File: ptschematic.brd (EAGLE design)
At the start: 33.5 x 51.6 mm, 26 parts, among them U3 NCP1117LPST33T3G, U4 BGM13S, Y2 32MHz

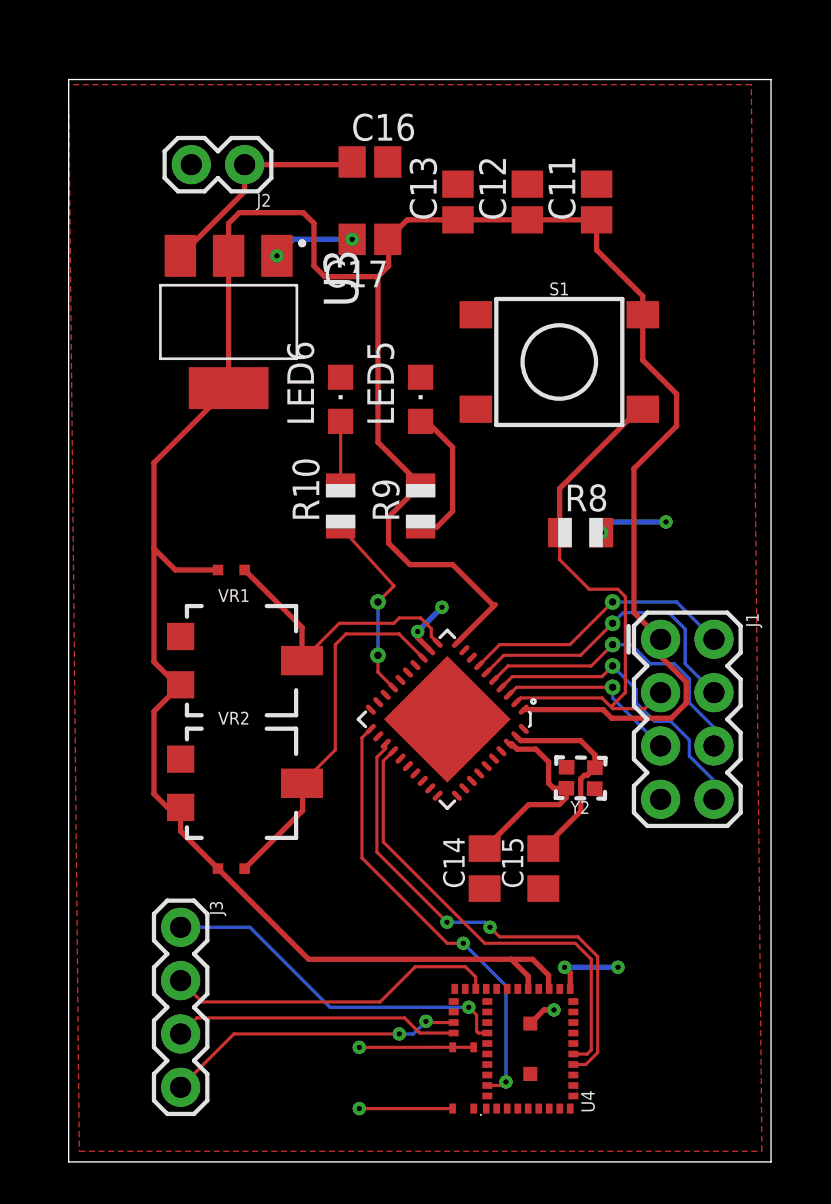
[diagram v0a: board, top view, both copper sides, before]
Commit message: Final Board and Gerber files
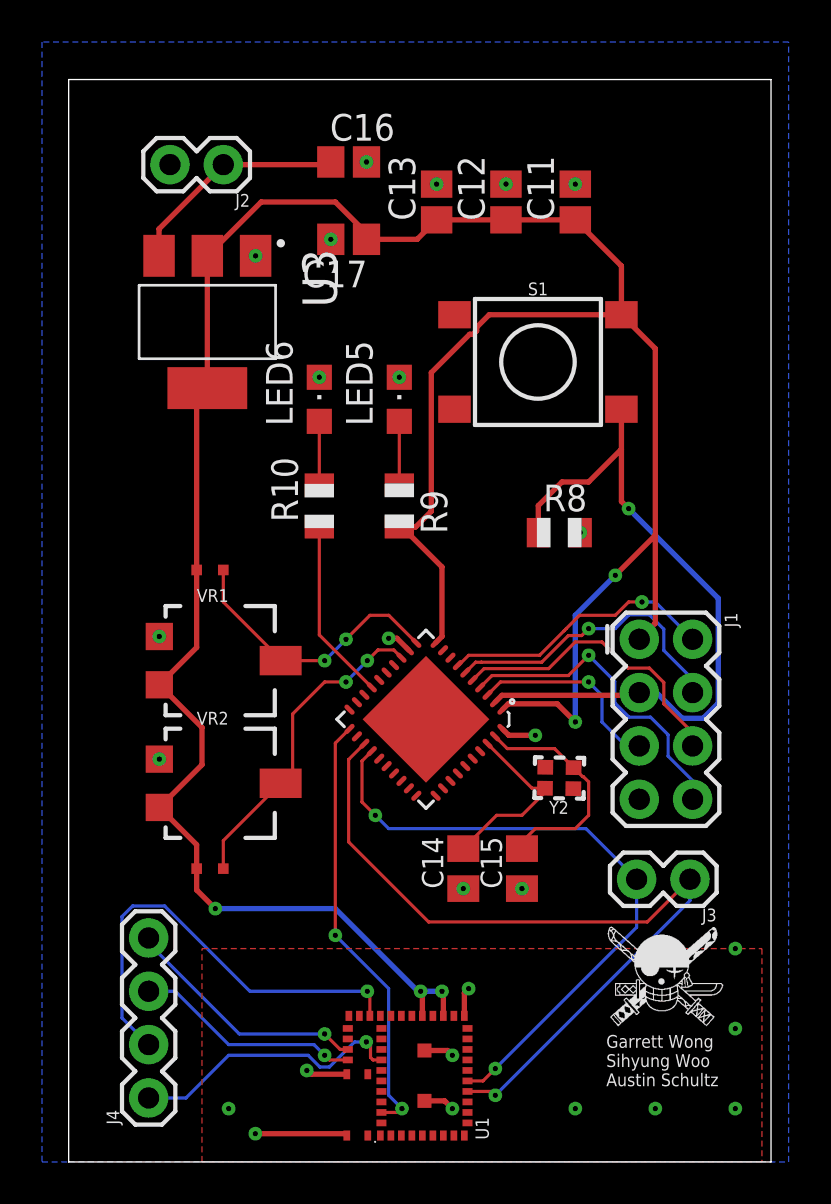
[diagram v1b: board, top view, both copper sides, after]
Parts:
- removed U4: BGM13S, BMES-Spr2019:BGM13S
- added J4: (no value), SparkFun-Connectors:1X04
- added U1: BGM13S, BMES-Spr2019:BGM13S
- J3: device SparkFun-Connectors:1X04 -> SparkFun-Connectors:1X02
- moved J3 24.4 mm to (29.6, 13.5), turned to 180 degrees
- moved C11 1.02 mm to (24.1, 45.7)
- moved C12 1.02 mm to (20.8, 45.7)
- moved C13 1.02 mm to (17.5, 45.7)
- moved C14 1.02 mm to (18.8, 14.0)
- moved C15 1.02 mm to (21.6, 14.0)
- moved R8 1.02 mm to (23.4, 30.0)
- moved Y2 1.02 mm to (23.4, 18.3)
- moved C16 1.02 mm to (13.3, 47.6)
- moved C17 1.02 mm to (13.3, 43.9)
- moved J2 1.02 mm to (7.37, 47.5)
- moved LED5 1.02 mm to (15.7, 36.3)
- moved LED6 1.02 mm to (11.9, 36.3)
- moved R10 1.02 mm to (11.9, 31.2)
- moved R9 1.02 mm to (15.7, 31.2), turned to 270 degrees
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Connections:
- removed net N$1: J3.4, U4.P$34
- removed net N$2: J3.3, U4.P$35
- removed net N$3: J3.2, U4.P$29
- removed net N$4: J3.1, U4.P$39
- new net N$5: J4.4, U1.P$34
- new net N$6: J4.3, U1.P$35
- new net N$7: J4.2, U1.P$29
- new net N$8: J4.1, U1.P$39
- net 1V8: now also U1.P$23; no longer U4.P$23
- net 3.3V: now also U1.P$22, U1.P$24; no longer U4.P$22, U4.P$24
- net A1RXD: now also J3.1, U1.P$13; no longer U4.P$13
- net A1TXD: now also J3.2, U1.P$14; no longer U4.P$14
- net BGMRST: now also U1.P$44; no longer U4.P$44
- net GND: now also U1.P$1, U1.P$2, U1.P$20, U1.P$3, U1.P$31, U1.P$4, U1.P$45, U1.P$46, U1.P$47, U1.P$48, U1.P$49, U1.P$5, U1.P$50, U1.P$51; no longer U4.P$1, U4.P$2, U4.P$20, U4.P$3, U4.P$31, U4.P$4, U4.P$45, U4.P$46, U4.P$47, U4.P$48, U4.P$49, U4.P$5, U4.P$50, U4.P$51
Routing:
- net N$7: track 0.00 -> 21.4 mm, vias 0 -> 1
- net N$4: track 17.1 -> 0.00 mm
- net N$3: track 15.9 -> 0.00 mm, vias 0 -> 1
- net A1RXD: track 23.9 -> 39.2 mm, vias 2 -> 1
- net N$1: track 14.3 -> 0.00 mm, vias 2 -> 0
- net N$2: track 13.6 -> 0.00 mm, vias 0 -> 1
- net N$8: track 0.00 -> 13.3 mm, vias 0 -> 1
- net N$5: track 0.00 -> 11.8 mm, vias 0 -> 1
- net GND: track 24.9 -> 13.6 mm, vias 11 -> 20
- net N$6: track 0.00 -> 10.8 mm, vias 0 -> 1
- net A1TXD: track 22.0 -> 30.6 mm, vias 0 -> 2
- net RST: track 25.8 -> 33.9 mm, vias 0 -> 1
- net 3.3V: track 138.5 -> 131.0 mm, vias 0 -> 5
- net N$10: track 6.92 -> 3.03 mm
- net ADC2: track 17.4 -> 15.3 mm, vias 0 -> 2
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- added copper zone on layer 16, net GND
